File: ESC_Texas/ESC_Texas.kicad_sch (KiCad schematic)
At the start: 29 parts, among them IC1 nRF52840-QFAA-F-R7, J1 Conn_01x10_Pin, J11 Conn_01x01_Pin, J12 Conn_01x05_Pin, J13 Conn_01x06_Pin, J2 Conn_01x05_Pin, J3 Motor, J4 Conn_01x05_Pin, Y1 CM7V-T1A-32.768kHz, Y2 32MHz

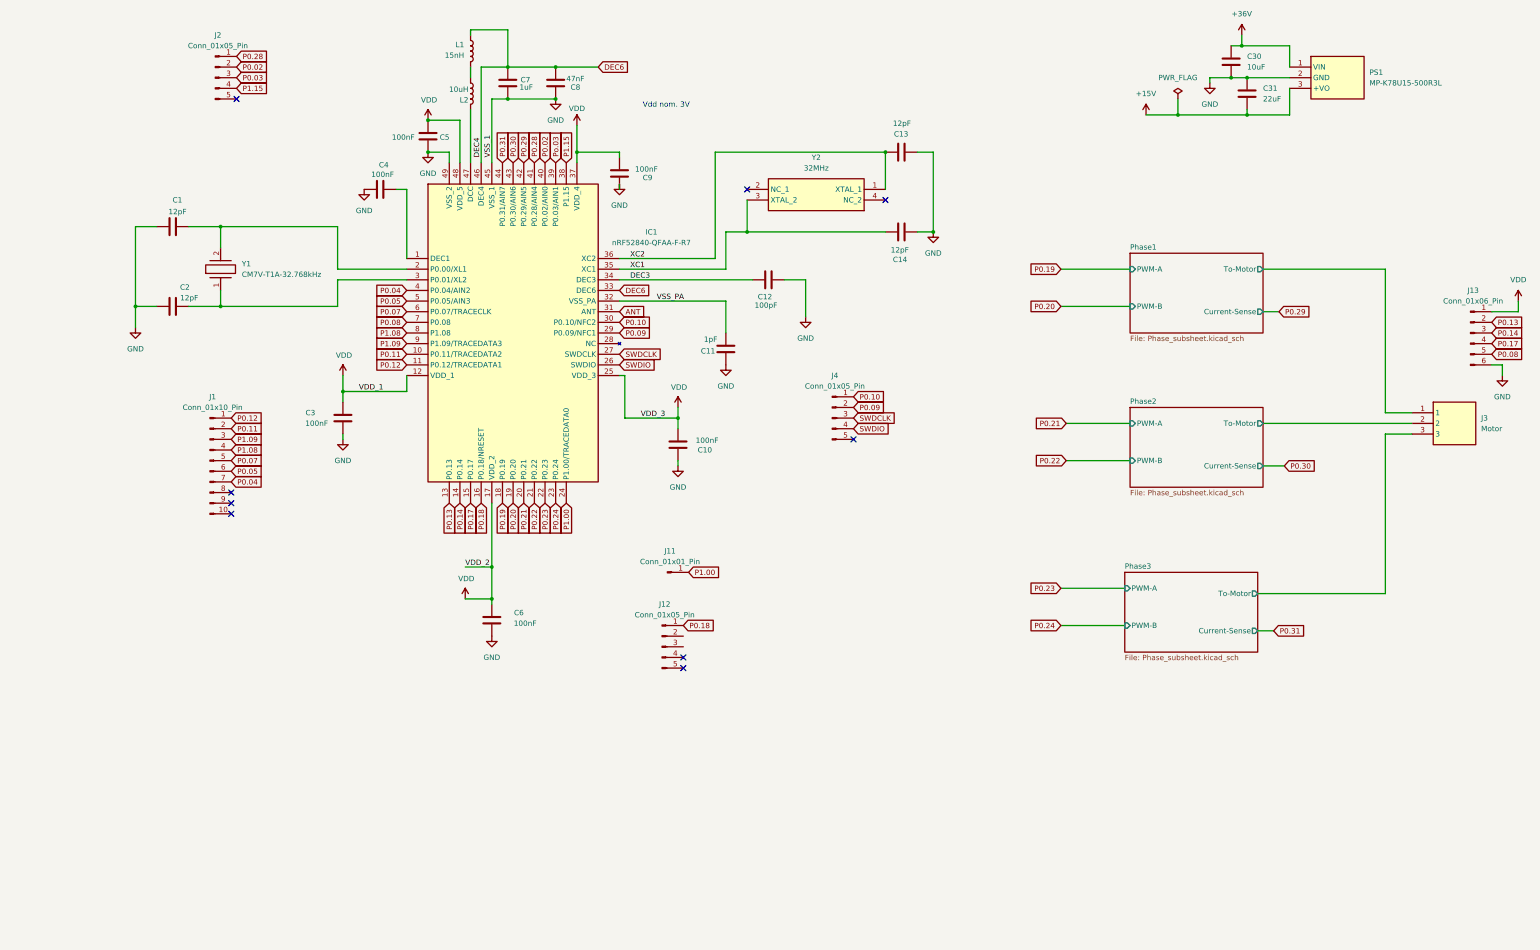
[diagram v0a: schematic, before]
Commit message: More routing done
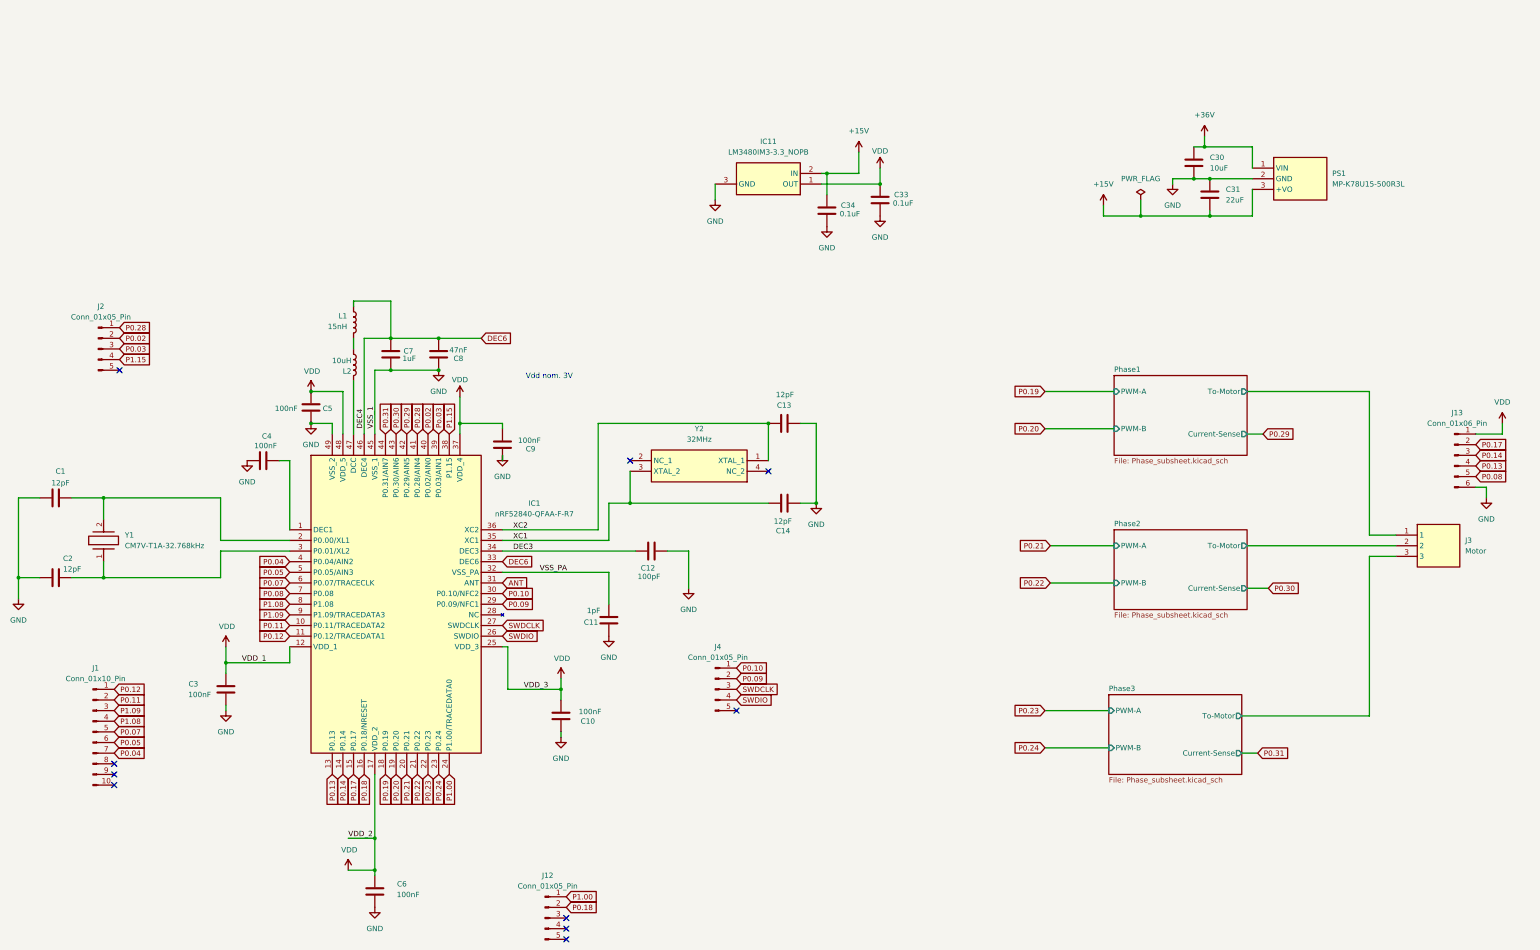
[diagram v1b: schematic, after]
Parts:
- removed J11: Conn_01x01_Pin, Connector_PinHeader_2.54mm:PinHeader_1x01_P2.54mm_Vertical, symbol Connector:Conn_01x01_Pin
- added C33, C34: 0.1uF, Capacitor_SMD:C_0805_2012Metric, symbol Device:C
- added IC11: LM3480IM3-3.3_NOPB, LM3480IM3-3.3_NOPB:SOT95P237X112-3N, symbol LM3480IM3-3_3_NOPB:LM3480IM3-3.3_NOPB
- C30, C31: footprint (none) -> Capacitor_SMD:C_0805_2012Metric
- J13: footprint (none) -> Connector_PinHeader_2.54mm:PinHeader_1x06_P2.54mm_Vertical
- J3: footprint SHDRRA3W90P0X350_1X3_1110X920X691P -> LIB_2350514-3:SHDRRA3W90P0X350_1X3_1110X920X691P
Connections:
- net +15V: now also C34.1, IC11.2 (IN)
- net GND: now also C33.2, C34.2, IC11.3 (GND)
- net P0.13: now also J13.4 (Pin_4); no longer J13.2 (Pin_2)
- net P0.17: now also J13.2 (Pin_2); no longer J13.4 (Pin_4)
- net P0.18: now also J12.2 (Pin_2); no longer J12.1 (Pin_1)
- net P1.00: now also J12.1 (Pin_1)
- net VDD: now also C33.1, IC11.1 (OUT)
- no-connect marks 9 -> 10
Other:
- moved on the sheet: C1, C10, C11, C12, C13, C14, C2, C3, C30, C31, C4, C5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
